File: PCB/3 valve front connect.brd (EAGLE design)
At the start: 83.2 x 35.2 mm, 17 parts, among them T1 2N2222, T2 2N2222, T3 2N2222

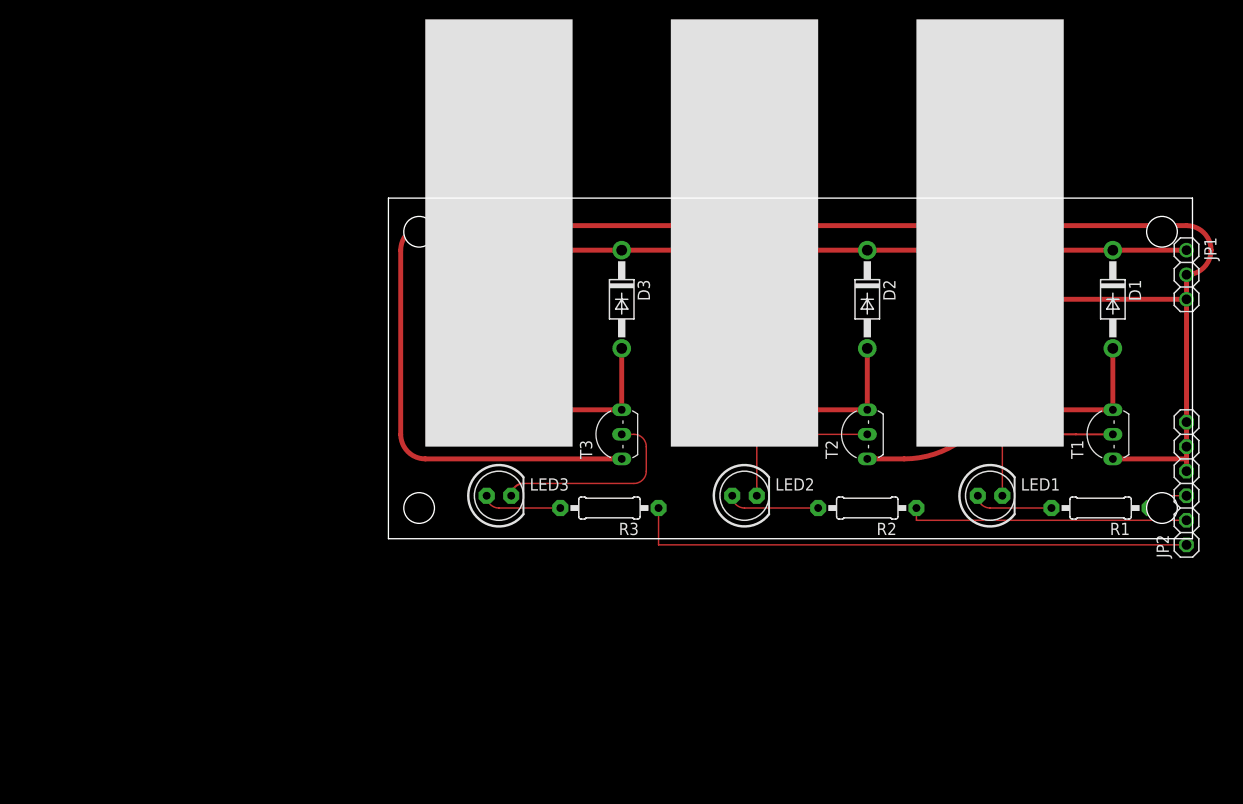
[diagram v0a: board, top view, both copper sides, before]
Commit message: board updates
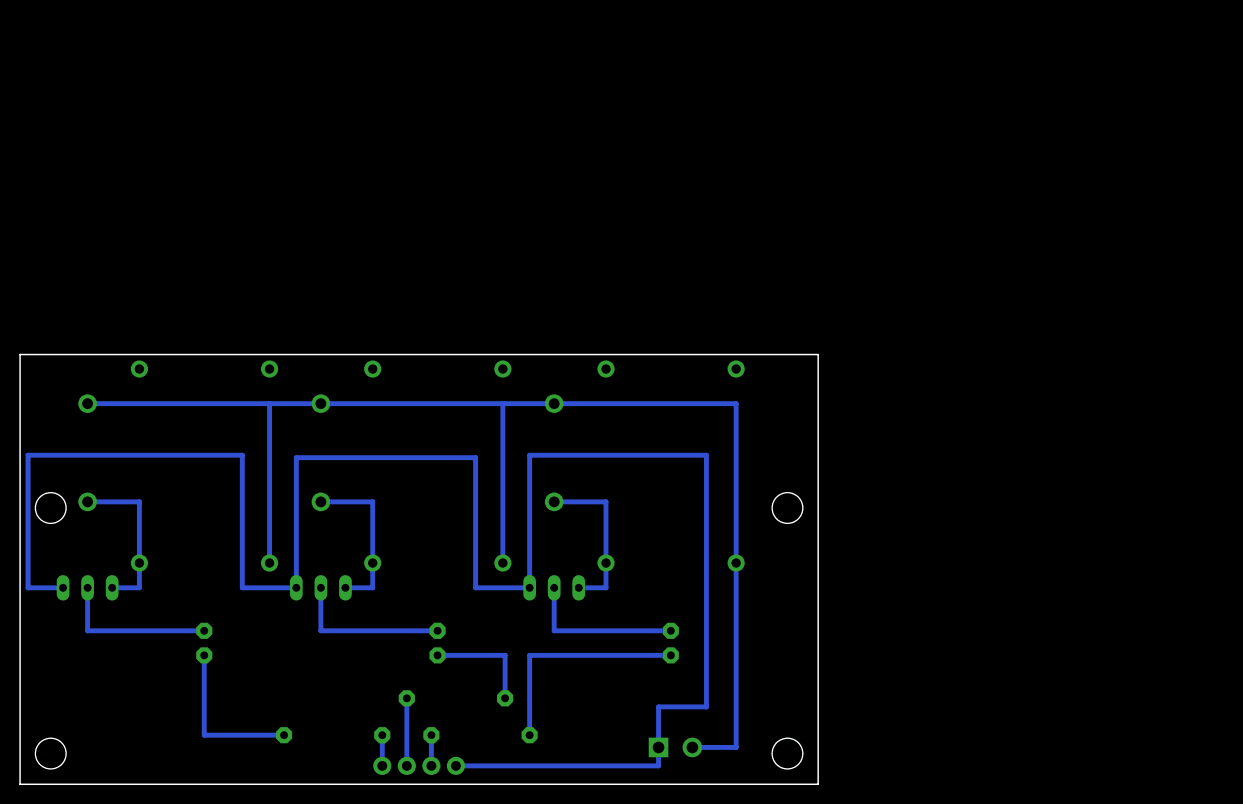
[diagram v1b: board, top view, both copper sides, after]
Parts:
- removed JP1: (no value), adafruit:1X03
- removed JP2: (no value), adafruit:1X06
- removed U$3: (no value), local eagle library:VALVTEST2
- added J1: (no value), SparkFun-Connectors:SCREWTERMINAL-3.5MM-2
- added SV1: (no value), SparkFun-Connectors:1X04
- added VALVE3: (no value), local eagle library:VALVTEST2
- moved R1 68.3 mm to (3.17, 5.08), flipped to the bottom
- moved D1 59.9 mm to (10.8, 34.3), flipped to the bottom
- moved T1 59.1 mm to (10.8, 19.1), flipped to the bottom, turned to 180 degrees
- moved D2 58.7 mm to (-13.3, 34.3), flipped to the bottom
- moved T2 57.8 mm to (-13.3, 19.1), flipped to the bottom, turned to 180 degrees
- moved D3 57.5 mm to (-37.5, 34.3), flipped to the bottom
- moved T3 56.6 mm to (-37.5, 19.1), flipped to the bottom, turned to 180 degrees
- moved R2 46.9 mm to (0.64, 8.89), flipped to the bottom
- moved R3 37.0 mm to (-12.1, 5.08), flipped to the bottom, turned to 0 degrees
- moved U$1 36.6 mm to (30.5, 19.1), flipped to the bottom
- moved LED1 36.4 mm to (22.9, 14.6), flipped to the bottom, turned to 90 degrees
- moved U$2 35.5 mm to (6.35, 19.1), flipped to the bottom
- moved LED2 35.2 mm to (-1.27, 14.6), flipped to the bottom, turned to 90 degrees
- moved LED3 34.1 mm to (-25.4, 14.6), flipped to the bottom, turned to 90 degrees
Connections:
- removed net VALVEGPIO1: JP2.3, R1.1
- removed net VALVEGPIO2: JP2.2, R2.1
- removed net VALVEGPIO3: JP2.1, R3.1
- new net N$19: R3.1, SV1.1
- new net N$30: R1.1, SV1.3
- new net N$44: R2.1, SV1.2
- net 5V: now also J1.2, VALVE3.PAD10; no longer JP1.1, U$3.PAD10
- net GND: now also J1.1, SV1.4; no longer JP1.2, JP2.4
- net N$9: now also VALVE3.PAD11; no longer U$3.PAD11
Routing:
- net VALVEGPIO3: track 58.4 -> 0.00 mm
- net VALVEGPIO2: track 29.2 -> 0.00 mm
- net 5V: track 125.0 -> 140.1 mm
- net N$3: track 8.15 -> 22.9 mm
- net N$11: track 8.25 -> 16.5 mm
- net N$44: track 0.00 -> 6.99 mm
- net N$5: track 12.4 -> 17.1 mm
- net N$1: track 12.4 -> 17.1 mm
- net VALVEGPIO1: track 4.34 -> 0.00 mm
- net N$9: track 12.9 -> 17.1 mm
- net N$10: track 20.6 -> 16.5 mm
- net GND: track 203.3 -> 199.9 mm
- net N$30: track 0.00 -> 3.17 mm
- net N$19: track 0.00 -> 3.17 mm
- net N$7: track 9.42 -> 11.4 mm
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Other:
- board size 83.2 x 35.2 mm -> 82.6 x 44.5 mm
